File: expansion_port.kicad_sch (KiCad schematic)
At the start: 1 part, among them J2 Conn_02x30_Odd_Even

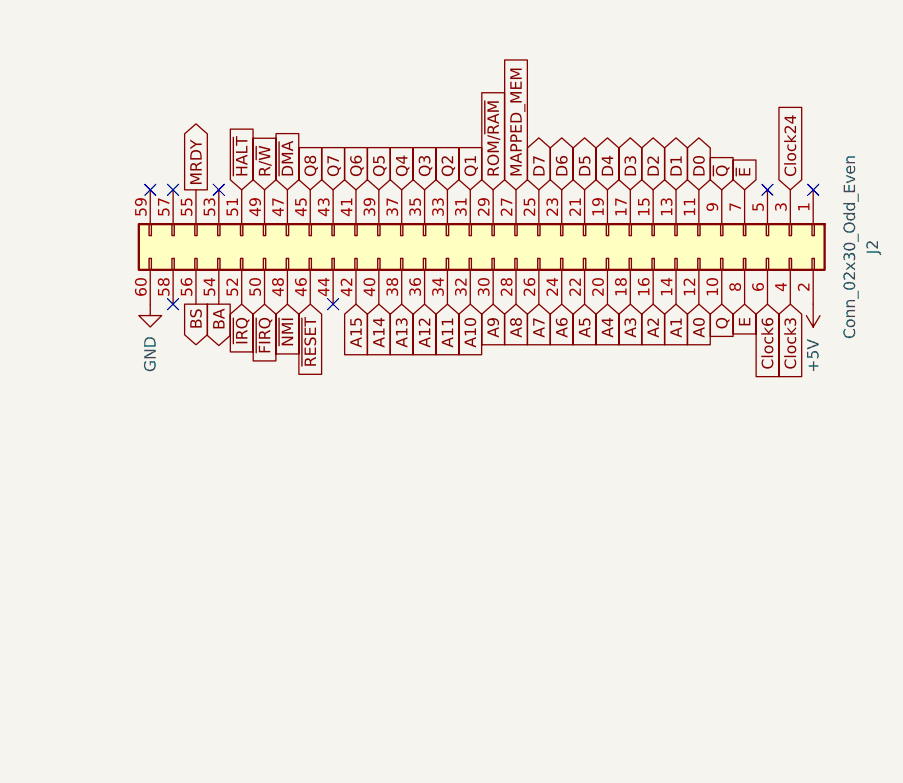
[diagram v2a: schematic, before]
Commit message: convert to new format
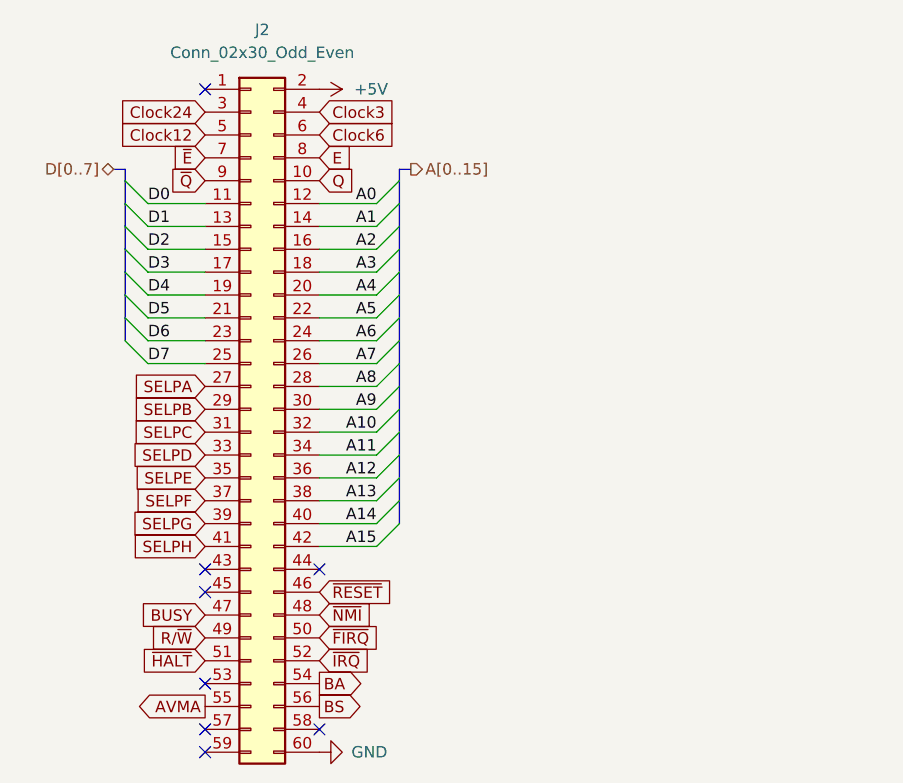
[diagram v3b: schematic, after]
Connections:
- net Clock12: now reaches J2.5 (Pin_5)
- net MAPPED_MEM renamed SELPA
- net MRDY renamed AVMA
- net Q1 renamed SELPC
- net Q2 renamed SELPD
- net Q3 renamed SELPE
- net Q4 renamed SELPF
- net Q5 renamed SELPG
- net Q6 renamed SELPH
- net Q7: no longer names the net of J2.43 (Pin_43)
- net Q8: no longer names the net of J2.45 (Pin_45)
- net ROM/~{RAM} renamed SELPB
- net ~{DMA} renamed BUSY
- no-connect marks 7 -> 8
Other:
- title: (none) -> HD6309 Homebrew SBC
- moved on the sheet: J2
